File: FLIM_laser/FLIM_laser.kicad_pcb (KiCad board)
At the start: 2 copper layers, 28.6 x 25 mm, 24 parts, among them J1 Conn_01x02_Male, J2 Conn_01x02_Male, J3 Conn_01x02_Male, J4 Conn_01x02_Male, M1 EP2014C, U1 AMS1117-5.0, U2 LMG1020, U3 74LVC1G08

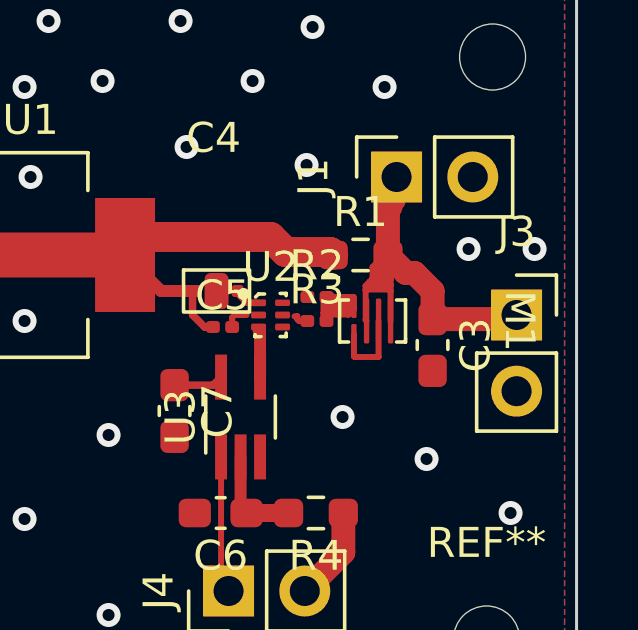
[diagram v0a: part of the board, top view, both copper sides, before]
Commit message: v0.94 something
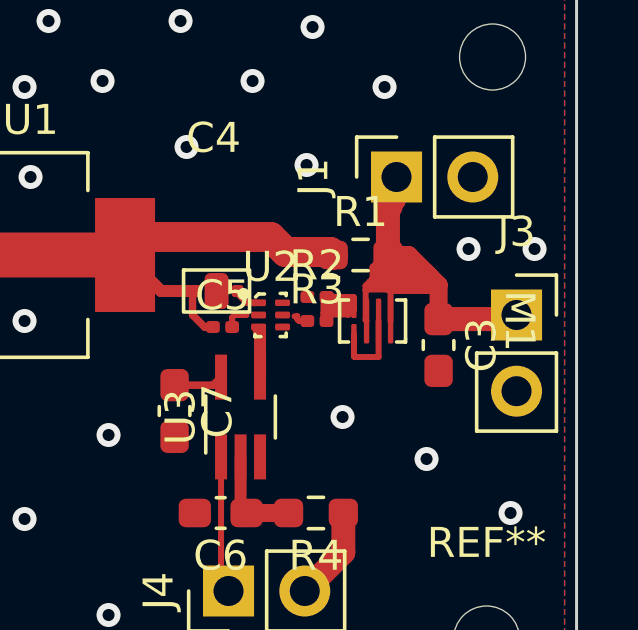
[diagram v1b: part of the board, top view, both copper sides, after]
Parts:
- moved C3 0.20 mm to (169.6, 51.0)
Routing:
- net Net-(C3-Pad1): track 18.8 -> 22.5 mm
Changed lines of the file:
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@@
   )
   (footprint "Capacitor_SMD:C_0603_1608Metric_Pad1.08x0.95mm_HandSolder" (layer "F.Cu")
-    (at 169.4 51 -90)
+    (at 169.6 51 -90)
     (descr "Capacitor SMD 0603 (1608 Metric), square (rectangular) end terminal, IPC_7351 nominal with elongated pad for handsoldering. (Body size source: IPC-SM-782 page 76, https://www.pcb-3d.com/wordpress/wp-content/uploads/ipc-sm-782a_amendment_1_and_2.pdf), generated with kicad-footprint-generator")
     (tags "capacitor handsolder")
@@
   (segment (start 166.6 49.8) (end 166.2 49.8) (width 0.3) (layer "F.Cu") (net 9))
   (segment (start 167.8 48.6) (end 167.8 48.8) (width 0.2) (layer "F.Cu") (net 10))
+  (segment (start 167.8 48.6) (end 169.2 48.6) (width 0.6) (layer "F.Cu") (net 10))
   (segment (start 168 49) (end 168 48.8) (width 0.2) (layer "F.Cu") (net 10))
   (segment (start 167.8 48.1125) (end 167.9125 48) (width 0.2) (layer "F.Cu") (net 10))
+  (segment (start 169.6 50.1375) (end 172.0625 50.1375) (width 0.8) (layer "F.Cu") (net 10))
   (segment (start 168.2 45.4) (end 168.2 46.2) (width 0.6) (layer "F.Cu") (net 10))
   (segment (start 167.9125 48) (end 167.9125 48.0875) (width 0.2) (layer "F.Cu") (net 10))
@@
   (segment (start 167.6 48.6) (end 167.8 48.6) (width 0.2) (layer "F.Cu") (net 10))
   (segment (start 168.2 46.2) (end 168 46.4) (width 0.6) (layer "F.Cu") (net 10))
-  (segment (start 168.8 48.6) (end 169.4 49.2) (width 0.8) (layer "F.Cu") (net 10))
+  (segment (start 172.0625 50.1375) (end 172.2 50) (width 0.8) (layer "F.Cu") (net 10))
   (segment (start 167.9125 48.0875) (end 167.6 48.4) (width 0.2) (layer "F.Cu") (net 10))
+  (segment (start 167.9125 48) (end 167.9125 48.45) (width 0.8) (layer "F.Cu") (net 10))
   (segment (start 167.4 49) (end 168 49) (width 0.2) (layer "F.Cu") (net 10))
   (segment (start 167.4 48.8) (end 167.4 48.4) (width 0.2) (layer "F.Cu") (net 10))
+  (segment (start 168 49) (end 169.6 49) (width 0.6) (layer "F.Cu") (net 10))
   (segment (start 167.18856 49.15048) (end 167.95048 49.15048) (width 0.2) (layer "F.Cu") (net 10))
   (segment (start 168 48.8) (end 167.8 48.8) (width 0.2) (layer "F.Cu") (net 10))
+  (segment (start 169.6 49) (end 169.6 50.1375) (width 0.6) (layer "F.Cu") (net 10))
   (segment (start 167.95048 49.15048) (end 168 49.2) (width 0.2) (layer "F.Cu") (net 10))
   (segment (start 168 50.2) (end 168 49.2) (width 0.2) (layer "F.Cu") (net 10))
@@
   (segment (start 167.6 48.6) (end 167.4 48.8) (width 0.2) (layer "F.Cu") (net 10))
   (segment (start 167.16952 49.16952) (end 167.18856 49.15048) (width 0.2) (layer "F.Cu") (net 10))
-  (segment (start 168.5125 48.6) (end 168.8 48.6) (width 0.8) (layer "F.Cu") (net 10))
-  (segment (start 169.4 50.1375) (end 172.0625 50.1375) (width 0.8) (layer "F.Cu") (net 10))
   (segment (start 168 49.2) (end 168 49) (width 0.2) (layer "F.Cu") (net 10))
   (segment (start 167.16952 50.16952) (end 167.2 50.2) (width 0.2) (layer "F.Cu") (net 10))
   (segment (start 168 46.4) (end 167.9125 46.4875) (width 0.8) (layer "F.Cu") (net 10))
   (segment (start 167.4 48.8) (end 167.3 48.9) (width 0.2) (layer "F.Cu") (net 10))
-  (segment (start 167.9125 48) (end 168.5125 48.6) (width 0.8) (layer "F.Cu") (net 10))
   (segment (start 167.8 48.8) (end 167.4 48.8) (width 0.2) (layer "F.Cu") (net 10))
   (segment (start 167.3 48.9) (end 167.4 49) (width 0.2) (layer "F.Cu") (net 10))
   (segment (start 167.3 48.9) (end 167.16952 49.03048) (width 0.2) (layer "F.Cu") (net 10))
-  (segment (start 172.0625 50.1375) (end 172.2 50) (width 0.8) (layer "F.Cu") (net 10))
+  (segment (start 168.6 48) (end 169.3 48.7) (width 0.6) (layer "F.Cu") (net 10))
   (segment (start 167.9125 48.4875) (end 167.8 48.6) (width 0.2) (layer "F.Cu") (net 10))
+  (segment (start 167.9125 48) (end 168.6 48) (width 0.6) (layer "F.Cu") (net 10))
+  (segment (start 169.3 48.7) (end 169.6 49) (width 0.6) (layer "F.Cu") (net 10))
   (segment (start 167.16952 49.03048) (end 167.16952 49.16952) (width 0.2) (layer "F.Cu") (net 10))
   (segment (start 168 48.0875) (end 167.9125 48) (width 0.2) (layer "F.Cu") (net 10))
@@
   (segment (start 167.9125 46.4875) (end 167.9125 48) (width 0.8) (layer "F.Cu") (net 10))
   (segment (start 167.4 48.4) (end 167.8 48) (width 0.2) (layer "F.Cu") (net 10))
-  (segment (start 169.4 49.2) (end 169.4 50.1375) (width 0.8) (layer "F.Cu") (net 10))
   (segment (start 168 48.8) (end 168 48.0875) (width 0.2) (layer "F.Cu") (net 10))
+  (segment (start 169.2 48.6) (end 169.3 48.7) (width 0.6) (layer "F.Cu") (net 10))
   (segment (start 164.892011 50.042989) (end 164.797891 50.042989) (width 0.2) (layer "F.Cu") (net 11))
   (segment (start 164.954902 50.2) (end 164.892011 50.137109) (width 0.2) (layer "F.Cu") (net 11))
